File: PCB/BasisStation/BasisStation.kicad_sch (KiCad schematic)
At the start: 20 parts, among them SW1 SW_SPST, SW4 RESET_BUTTON, U2 ESP32-S3-WROOM-2, X4 JTAG

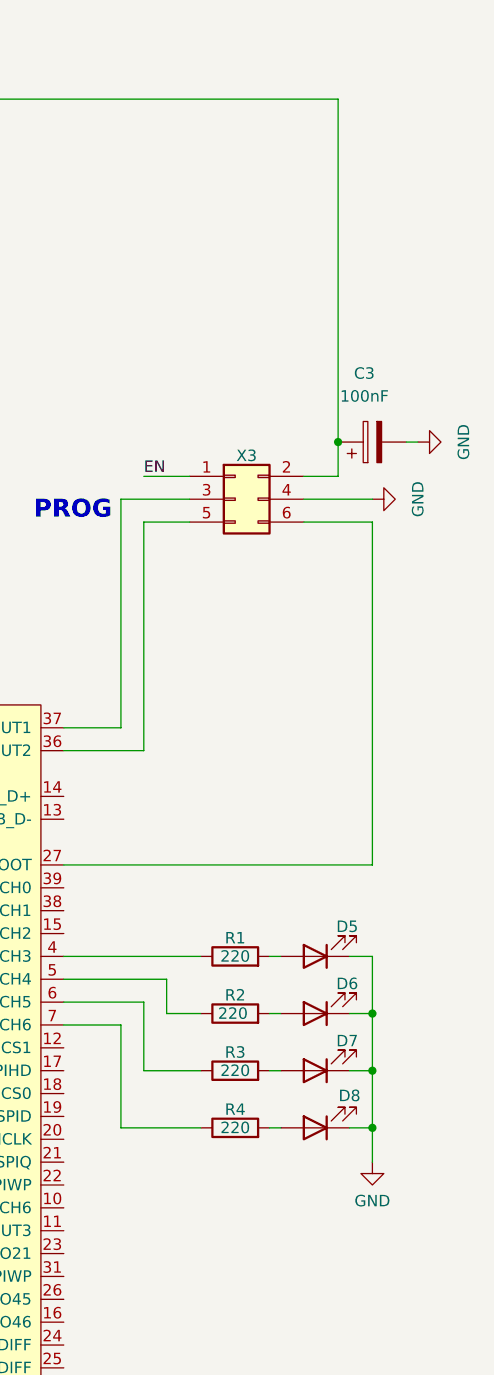
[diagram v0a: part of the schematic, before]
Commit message: PCB überarbeitet
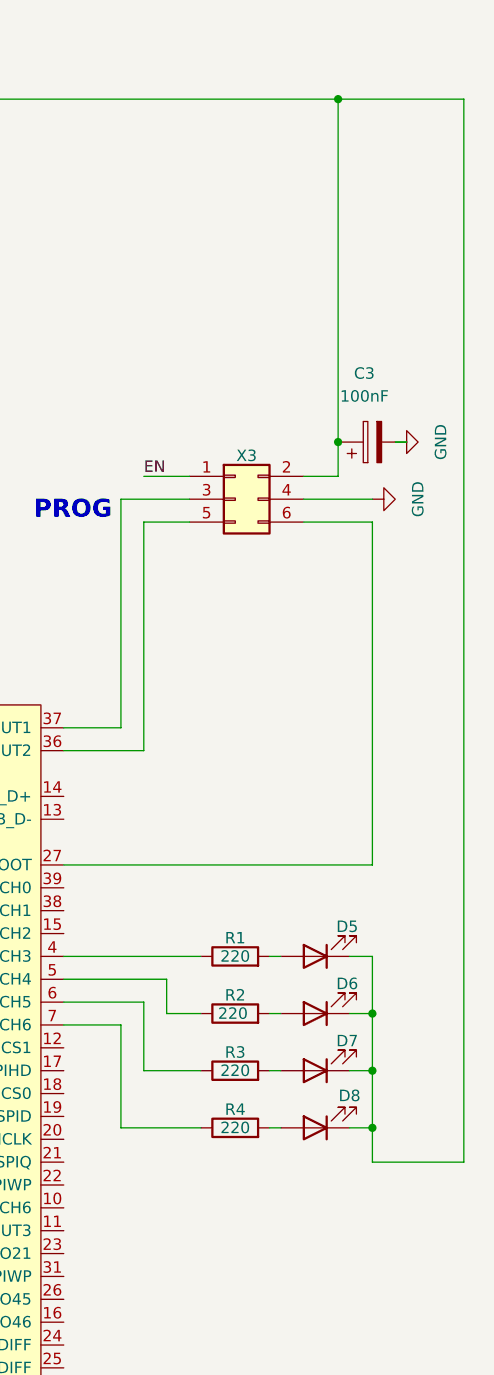
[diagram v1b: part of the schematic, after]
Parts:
- SW1: footprint CUSTOM_Footprint:WUE_SW_471001264143_2_00-3_00_ -> (none)
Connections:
- net GND: no longer D5.1 (K), D6.1 (K), D7.1 (K), D8.1 (K)
- net at C1.1, C3.1, C7.1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: now also D5.1 (K), D6.1 (K), D7.1 (K), D8.1 (K)
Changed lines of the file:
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@@
+	)
+	(junction
+		(at 181.61 27.94)
+		(diameter 0)
+		(color 0 0 0 0)
 	)
 	(junction
@@
 	(wire
 		(pts
+			(xy 195.58 146.05) (xy 195.58 27.94)
+		)
+		(stroke
+			(width 0)
+			(type default)
+		)
+	)
+	(wire
+		(pts
 			(xy 38.1 274.32) (xy 38.1 276.86)
 		)
@@
 	(wire
 		(pts
+			(xy 195.58 27.94) (xy 181.61 27.94)
+		)
+		(stroke
+			(width 0)
+			(type default)
+		)
+	)
+	(wire
+		(pts
 			(xy 162.56 129.54) (xy 162.56 125.73)
 		)
@@
 	(wire
 		(pts
-			(xy 189.23 66.04) (xy 190.5 66.04)
+			(xy 189.23 66.04) (xy 187.96 66.04)
 		)
 		(stroke
@@
 		(pts
 			(xy 157.48 142.24) (xy 166.37 142.24)
+		)
+		(stroke
+			(width 0)
+			(type default)
+		)
+	)
+	(wire
+		(pts
+			(xy 185.42 146.05) (xy 195.58 146.05)
 		)
 		(stroke
@@
 	(symbol
 		(lib_id "power:GND")
-		(at 190.5 66.04 90)
+		(at 187.96 66.04 90)
 		(unit 1)
 		(exclude_from_sim no)
@@
 		(fields_autoplaced yes)
 		(property "Reference" "#PWR01"
-			(at 196.85 66.04 0)
+			(at 194.31 66.04 0)
 			(effects
 				(font
@@
 		)
 		(property "Value" "GND"
-			(at 195.58 66.04 0)
+			(at 193.04 66.04 0)
 			(effects
 				(font
@@
 		)
 		(property "Footprint" ""
-			(at 190.5 66.04 0)
+			(at 187.96 66.04 0)
 			(effects
 				(font
@@
 		)
 		(property "Datasheet" ""
-			(at 190.5 66.04 0)
+			(at 187.96 66.04 0)
 			(effects
 				(font
@@
 		)
 		(property "Description" "Power symbol creates a global label with name \"GND\" , ground"
-			(at 190.5 66.04 0)
+			(at 187.96 66.04 0)
 			(effects
 				(font
@@
 			)
 		)
-		(property "Footprint" "CUSTOM_Footprint:WUE_SW_471001264143_2_00-3_00_"
+		(property "Footprint" ""
 			(at 30.48 40.64 0)
 			(effects
@@
 					(unit 1)
 				)
-			)
-		)
-	)
-	(symbol
-		(lib_id "power:GND")
-		(at 185.42 146.05 0)
-		(unit 1)
-		(exclude_from_sim no)
-		(in_bom yes)
-		(on_board yes)
-		(dnp no)
-		(property "Reference" "#PWR03"
-			(at 185.42 152.4 0)
-			(effects
-				(font
-					(size 1.27 1.27)
-				)
-				(hide yes)
-			)
-		)
-		(property "Value" "GND"
-			(at 185.42 150.368 0)
-			(effects
-				(font
-					(size 1.27 1.27)
-				)
-			)
-		)
-		(property "Footprint" ""
-			(at 185.42 146.05 0)
-			(effects
-				(font
-					(size 1.27 1.27)
-				)
-				(hide yes)
-			)
-		)
-		(property "Datasheet" ""
-			(at 185.42 146.05 0)
-			(effects
-				(font
-					(size 1.27 1.27)
-				)
-				(hide yes)
-			)
-		)
-		(property "Description" "Power symbol creates a global label with name \"GND\" , ground"
-			(at 185.42 146.05 0)
-			(effects
-				(font
-					(size 1.27 1.27)
-				)
-				(hide yes)
-			)
-		)
-		(pin "1"
-		)
-		(instances
-			(project "BasisStation"
-				(path "/cc03a18a-a128-4e00-a998-441923eeacd1"
-					(reference "#PWR03")
-					(unit 1)
-				)
